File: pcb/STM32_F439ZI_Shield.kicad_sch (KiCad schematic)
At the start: 12 parts, among them K1 G6S-2, K2 G6S-2, U1 LM2904, U2 MAX3485

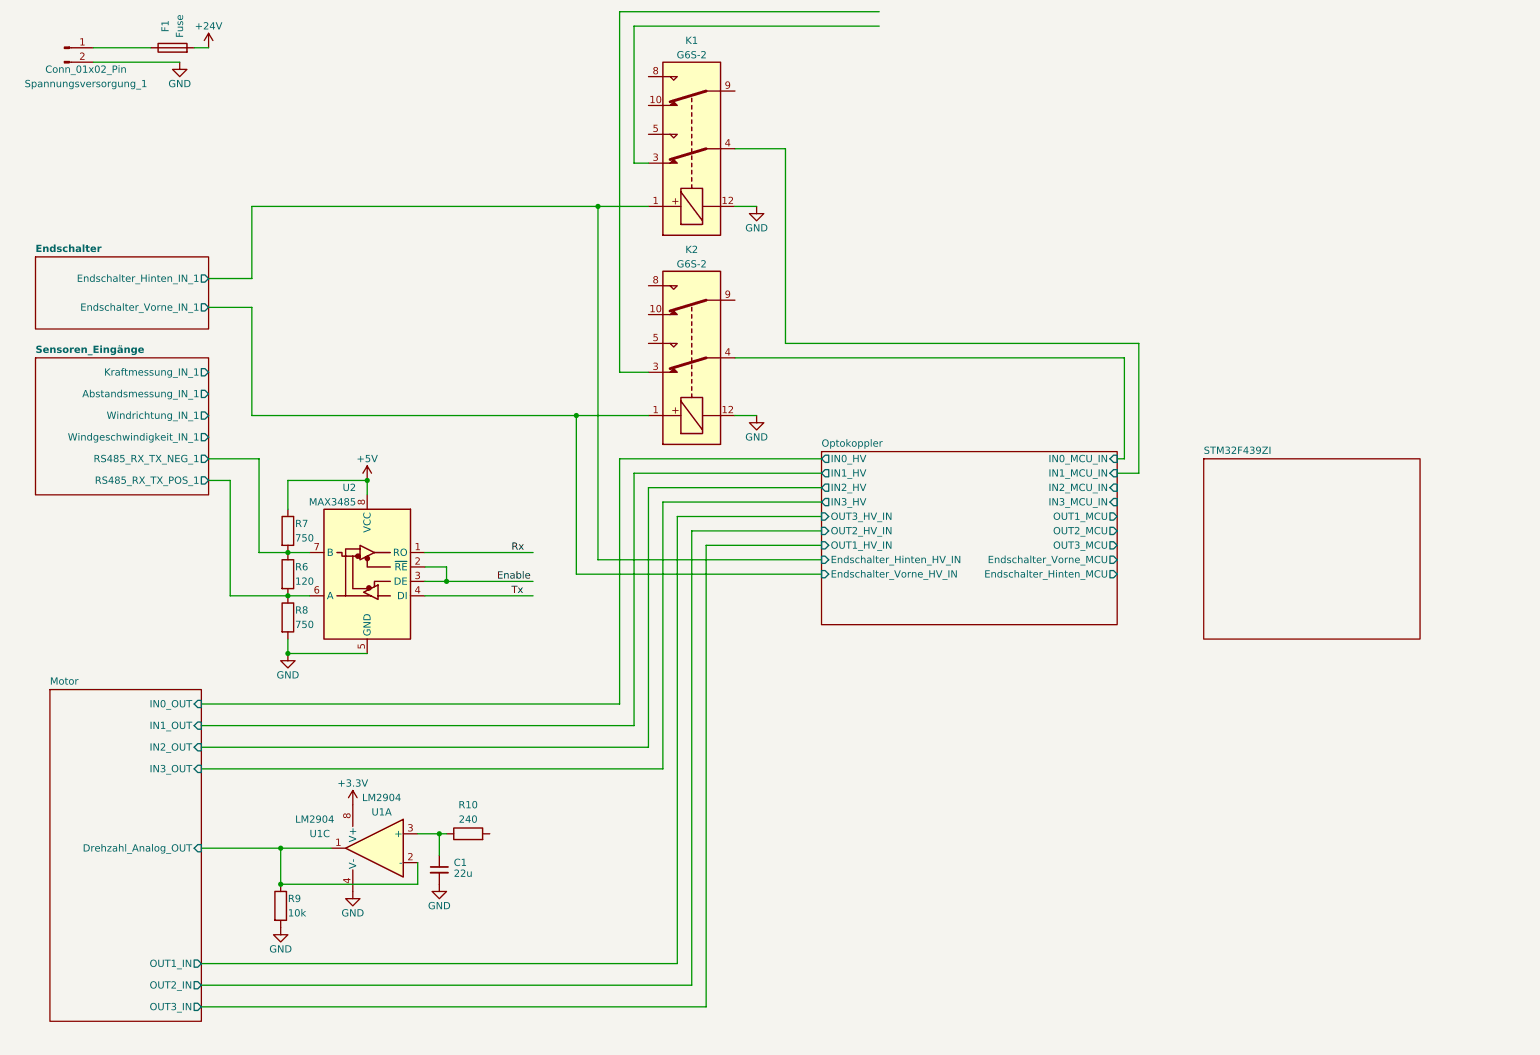
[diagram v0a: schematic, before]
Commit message: updated pcb
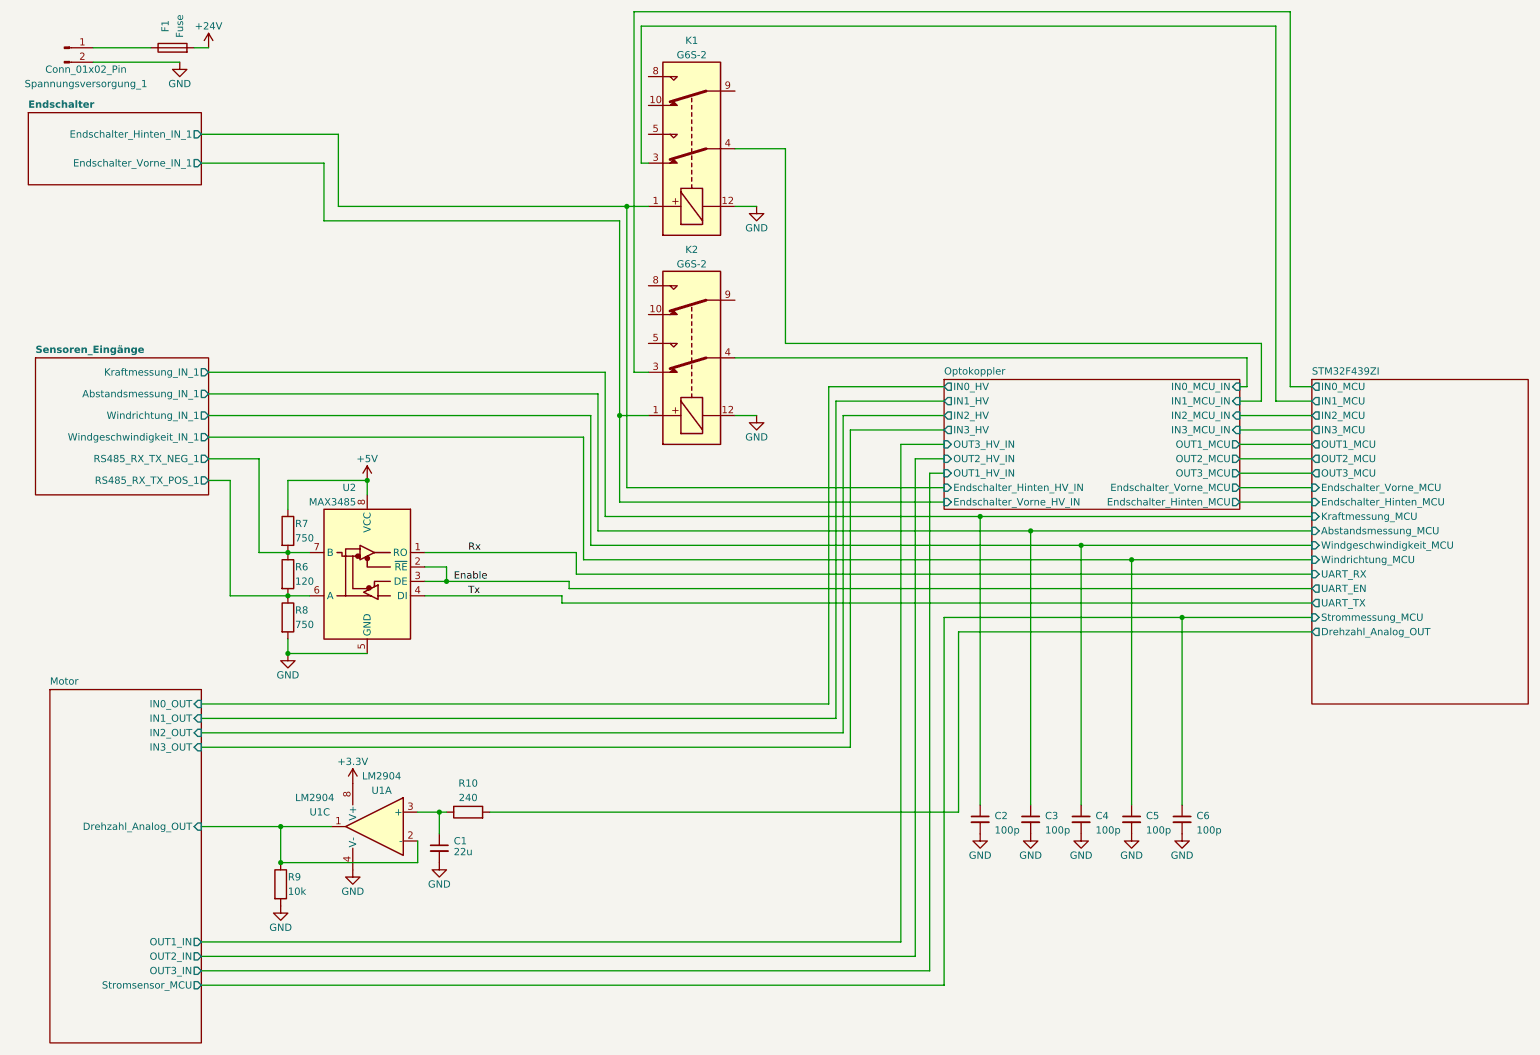
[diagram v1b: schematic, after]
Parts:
- added C2, C3, C4, C5, C6: 100p, Capacitor_SMD:C_0603_1608Metric, symbol Device:C_Small
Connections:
- net GND: now also C2.2, C3.2, C4.2, C5.2, C6.2
- net STM32F439ZI/IN0_MCU: now reaches K2.3
- net STM32F439ZI/IN1_MCU: now reaches K1.3
- net STM32F439ZI/Drehzahl_Analog_OUT: now reaches R10.2
- new net Motor/Stromsensor_MCU: C6.1
- new net STM32F439ZI/Abstandsmessung_MCU: C3.1
- new net STM32F439ZI/Kraftmessung_MCU: C2.1
- new net STM32F439ZI/Windgeschwindigkeit_MCU: C4.1
- new net STM32F439ZI/Windrichtung_MCU: C5.1
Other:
- sheet Motor ports: added Stromsensor_MCU; removed none
- sheet STM32F439ZI ports: added Abstandsmessung_MCU, Drehzahl_Analog_OUT, Endschalter_Hinten_MCU, Endschalter_Vorne_MCU, IN0_MCU, IN1_MCU, IN2_MCU, IN3_MCU, Kraftmessung_MCU, OUT1_MCU, OUT2_MCU, OUT3_MCU, Strommessung_MCU, UART_EN, UART_RX, UART_TX, Windgeschwindigkeit_MCU, Windrichtung_MCU; removed none
- moved on the sheet: C1, R10, R9, U1A, U1C
